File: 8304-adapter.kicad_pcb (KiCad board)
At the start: 2 copper layers, 16.5 x 27.9 mm, 4 parts, among them J2 Conn_01x10, J3 Conn_01x10, U1 74LS245

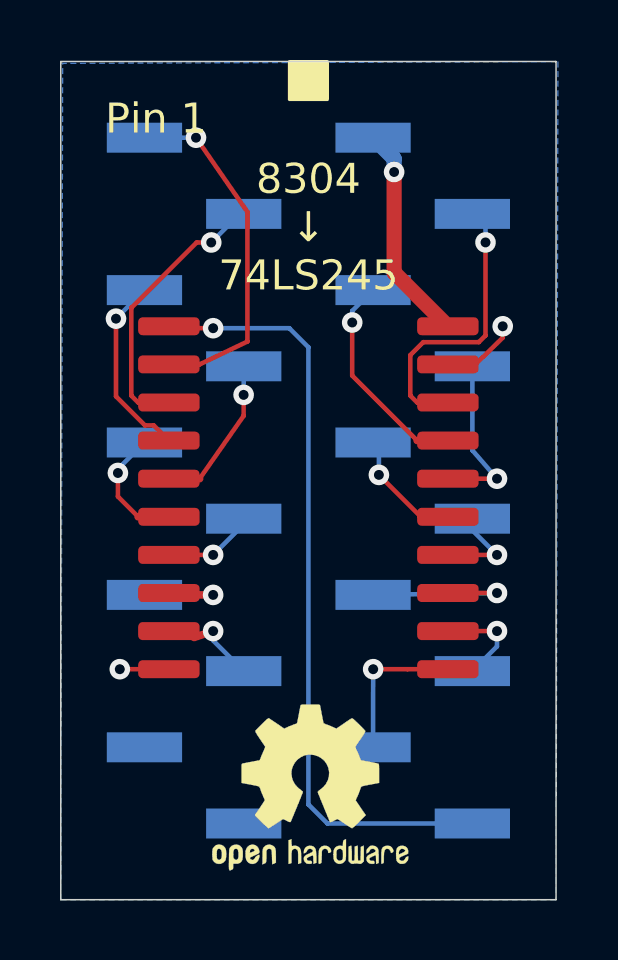
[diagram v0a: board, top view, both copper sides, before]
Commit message: Minor fixes
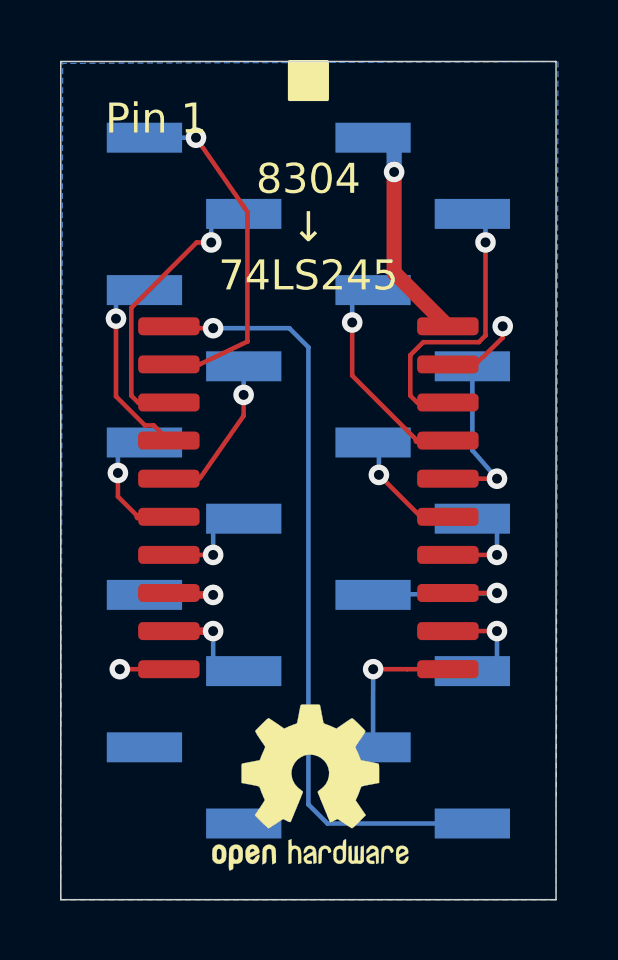
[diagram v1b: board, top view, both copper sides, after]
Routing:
- net A7: track 2.42 -> 3.52 mm
- net A3: track 5.23 -> 4.21 mm
- net A5: track 3.10 -> 3.70 mm
- net A1: track 9.32 -> 9.88 mm
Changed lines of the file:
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@@
     (thickness 1.6)
     (drawings 7)
-    (tracks 110)
+    (tracks 112)
     (zones 0)
     (modules 4)
@@
   (segment (start 45.72 24.765) (end 48.26 24.765) (width 0.1524) (layer B.Cu) (net 2))
   (via (at 45.72 24.765) (size 0.6858) (drill 0.3302) (layers F.Cu B.Cu) (net 2))
-  (segment (start 46.74 20.955) (end 46.609 20.955) (width 0.1524) (layer B.Cu) (net 3))
-  (segment (start 46.609 20.955) (end 45.6565 21.9075) (width 0.1524) (layer B.Cu) (net 3))
   (segment (start 45.6565 21.9075) (end 45.6565 21.9075) (width 0.1524) (layer B.Cu) (net 3))
   (via (at 45.6565 21.9075) (size 0.6858) (drill 0.3302) (layers F.Cu B.Cu) (net 3))
@@
   (segment (start 45.171567 21.9075) (end 42.99139 24.087677) (width 0.1524) (layer F.Cu) (net 3))
   (segment (start 45.6565 21.9075) (end 45.171567 21.9075) (width 0.1524) (layer F.Cu) (net 3))
+  (segment (start 45.6565 20.955) (end 45.6565 21.9075) (width 0.1524) (layer B.Cu) (net 3))
+  (segment (start 46.74 20.955) (end 45.6565 20.955) (width 0.1524) (layer B.Cu) (net 3))
   (segment (start 51.054 36.1315) (end 51.05 38.735) (width 0.1524) (layer B.Cu) (net 4))
   (via (at 51.054 36.1315) (size 0.6858) (drill 0.3302) (layers F.Cu B.Cu) (net 4))
@@
   (segment (start 44.245 28.5115) (end 43.736999 28.003499) (width 0.1524) (layer F.Cu) (net 5))
   (segment (start 42.4815 27.038436) (end 42.4815 24.511) (width 0.1524) (layer F.Cu) (net 5))
-  (segment (start 42.4815 24.4435) (end 43.43 23.495) (width 0.1524) (layer B.Cu) (net 5))
   (segment (start 42.4815 24.4475) (end 42.4815 24.4435) (width 0.1524) (layer B.Cu) (net 5))
+  (segment (start 42.799 23.495) (end 42.4815 23.8125) (width 0.1524) (layer B.Cu) (net 5))
+  (segment (start 43.43 23.495) (end 42.799 23.495) (width 0.1524) (layer B.Cu) (net 5))
+  (segment (start 42.4815 23.8125) (end 42.4815 23.749) (width 0.1524) (layer B.Cu) (net 5))
+  (segment (start 42.4815 24.4435) (end 42.4815 23.8125) (width 0.1524) (layer B.Cu) (net 5))
   (segment (start 53.9115 34.8615) (end 53.545 34.8615) (width 0.254) (layer F.Cu) (net 6))
   (segment (start 55.1815 34.8615) (end 53.9115 34.8615) (width 0.1524) (layer F.Cu) (net 6))
   (via (at 55.1815 34.8615) (size 0.6858) (drill 0.3302) (layers F.Cu B.Cu) (net 6))
-  (segment (start 55.1815 35.3735) (end 54.36 36.195) (width 0.1524) (layer B.Cu) (net 6))
-  (segment (start 55.1815 34.8615) (end 55.1815 35.3735) (width 0.1524) (layer B.Cu) (net 6))
-  (segment (start 45.27 29.7815) (end 44.245 29.7815) (width 0.254) (layer F.Cu) (net 7))
+  (segment (start 55.1815 35.8775) (end 54.36 36.195) (width 0.1524) (layer B.Cu) (net 6))
+  (segment (start 55.1815 34.8615) (end 55.1815 35.8775) (width 0.1524) (layer B.Cu) (net 6))
   (segment (start 46.74 26.3565) (end 46.74 26.035) (width 0.1524) (layer B.Cu) (net 7))
   (segment (start 46.736 26.9875) (end 46.74 26.3565) (width 0.1524) (layer B.Cu) (net 7))
@@
   (segment (start 42.545 29.591) (end 42.545 30.3765) (width 0.1524) (layer F.Cu) (net 9))
   (via (at 42.545 29.591) (size 0.6858) (drill 0.3302) (layers F.Cu B.Cu) (net 9))
-  (segment (start 42.545 29.46) (end 43.43 28.575) (width 0.1524) (layer B.Cu) (net 9))
-  (segment (start 42.545 29.591) (end 42.545 29.46) (width 0.1524) (layer B.Cu) (net 9))
+  (segment (start 42.545 28.956) (end 43.43 28.575) (width 0.1524) (layer B.Cu) (net 9))
+  (segment (start 42.545 29.591) (end 42.545 28.956) (width 0.1524) (layer B.Cu) (net 9))
   (segment (start 53.975 32.3215) (end 53.545 32.3215) (width 0.254) (layer F.Cu) (net 10))
   (segment (start 55.1815 32.3215) (end 53.975 32.3215) (width 0.1524) (layer F.Cu) (net 10))
   (via (at 55.1815 32.3215) (size 0.6858) (drill 0.3302) (layers F.Cu B.Cu) (net 10))
-  (segment (start 54.36 31.5) (end 54.36 31.115) (width 0.1524) (layer B.Cu) (net 10))
-  (segment (start 55.1815 32.3215) (end 54.36 31.5) (width 0.1524) (layer B.Cu) (net 10))
+  (segment (start 55.1815 31.4325) (end 54.36 31.115) (width 0.1524) (layer B.Cu) (net 10))
+  (segment (start 55.1815 32.3215) (end 55.1815 31.4325) (width 0.1524) (layer B.Cu) (net 10))
   (segment (start 44.245 32.3215) (end 45.72 32.3215) (width 0.1524) (layer F.Cu) (net 11))
   (segment (start 45.72 32.3215) (end 45.72 32.3215) (width 0.1524) (layer F.Cu) (net 11))
   (via (at 45.72 32.3215) (size 0.6858) (drill 0.3302) (layers F.Cu B.Cu) (net 11))
-  (segment (start 46.74 31.3015) (end 46.74 31.115) (width 0.1524) (layer B.Cu) (net 11))
-  (segment (start 45.72 32.3215) (end 46.74 31.3015) (width 0.1524) (layer B.Cu) (net 11))
+  (segment (start 45.72 31.115) (end 46.74 31.115) (width 0.1524) (layer B.Cu) (net 11))
+  (segment (start 45.72 32.3215) (end 45.72 31.115) (width 0.1524) (layer B.Cu) (net 11))
   (segment (start 52.6415 31.0515) (end 53.545 31.0515) (width 0.254) (layer F.Cu) (net 12))
   (segment (start 51.2445 29.6545) (end 52.6415 31.0515) (width 0.1524) (layer F.Cu) (net 12))
@@
   (via (at 55.1815 29.7815) (size 0.6858) (drill 0.3302) (layers F.Cu B.Cu) (net 14))
   (segment (start 55.1815 29.7815) (end 53.545 29.7815) (width 0.1524) (layer F.Cu) (net 14))
-  (segment (start 45.724 35.179) (end 46.74 36.195) (width 0.1524) (layer B.Cu) (net 15))
-  (segment (start 45.72 34.8615) (end 45.724 35.179) (width 0.1524) (layer B.Cu) (net 15))
-  (segment (start 45.72 34.8615) (end 45.085 35.075067) (width 0.254) (layer F.Cu) (net 15))
   (via (at 45.72 34.8615) (size 0.6858) (drill 0.3302) (layers F.Cu B.Cu) (net 15))
+  (segment (start 45.72 34.8615) (end 44.245 34.8615) (width 0.254) (layer F.Cu) (net 15))
+  (segment (start 45.72 35.814) (end 46.74 36.195) (width 0.1524) (layer B.Cu) (net 15))
+  (segment (start 45.72 34.8615) (end 45.72 35.814) (width 0.1524) (layer B.Cu) (net 15))
   (segment (start 52.52 28.5115) (end 53.545 28.5115) (width 0.254) (layer F.Cu) (net 16))
   (segment (start 50.3555 26.347) (end 52.52 28.5115) (width 0.1524) (layer F.Cu) (net 16))
   (segment (start 50.3555 24.5745) (end 50.3555 26.347) (width 0.1524) (layer F.Cu) (net 16))
   (via (at 50.3555 24.5745) (size 0.6858) (drill 0.3302) (layers F.Cu B.Cu) (net 16))
-  (segment (start 50.3555 24.1895) (end 51.05 23.495) (width 0.1524) (layer B.Cu) (net 16))
-  (segment (start 50.3555 24.5745) (end 50.3555 24.1895) (width 0.1524) (layer B.Cu) (net 16))
+  (segment (start 50.3555 23.495) (end 51.05 23.495) (width 0.1524) (layer B.Cu) (net 16))
+  (segment (start 50.3555 24.5745) (end 50.3555 23.495) (width 0.1524) (layer B.Cu) (net 16))
   (segment (start 52.52 27.2415) (end 53.545 27.2415) (width 0.1524) (layer F.Cu) (net 17))
   (segment (start 52.29139 27.01289) (end 52.52 27.2415) (width 0.1524) (layer F.Cu) (net 17))
@@
   (segment (start 55.372 25.0825) (end 54.462678 25.9715) (width 0.1524) (layer F.Cu) (net 18))
   (segment (start 55.372 24.7015) (end 55.372 25.0825) (width 0.1524) (layer F.Cu) (net 18))
-  (segment (start 51.7525 19.1175) (end 51.05 18.415) (width 0.508) (layer B.Cu) (net 19))
-  (segment (start 51.7525 19.558) (end 51.7525 19.1175) (width 0.508) (layer B.Cu) (net 19))
   (segment (start 51.7525 22.909) (end 53.545 24.7015) (width 0.508) (layer F.Cu) (net 19))
   (segment (start 51.7525 19.558) (end 51.7525 22.909) (width 0.508) (layer F.Cu) (net 19))
   (via (at 51.7525 19.558) (size 0.6858) (drill 0.3302) (layers F.Cu B.Cu) (net 19))
+  (segment (start 51.7525 18.7325) (end 51.05 18.415) (width 0.508) (layer B.Cu) (net 19))
+  (segment (start 51.7525 19.558) (end 51.7525 18.7325) (width 0.508) (layer B.Cu) (net 19))
   (zone (net 18) (net_name GND) (layer B.Cu) (hatch edge 0.508)
     (connect_pads (clearance 0.508))
